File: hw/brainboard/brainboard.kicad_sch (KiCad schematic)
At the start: 0 parts

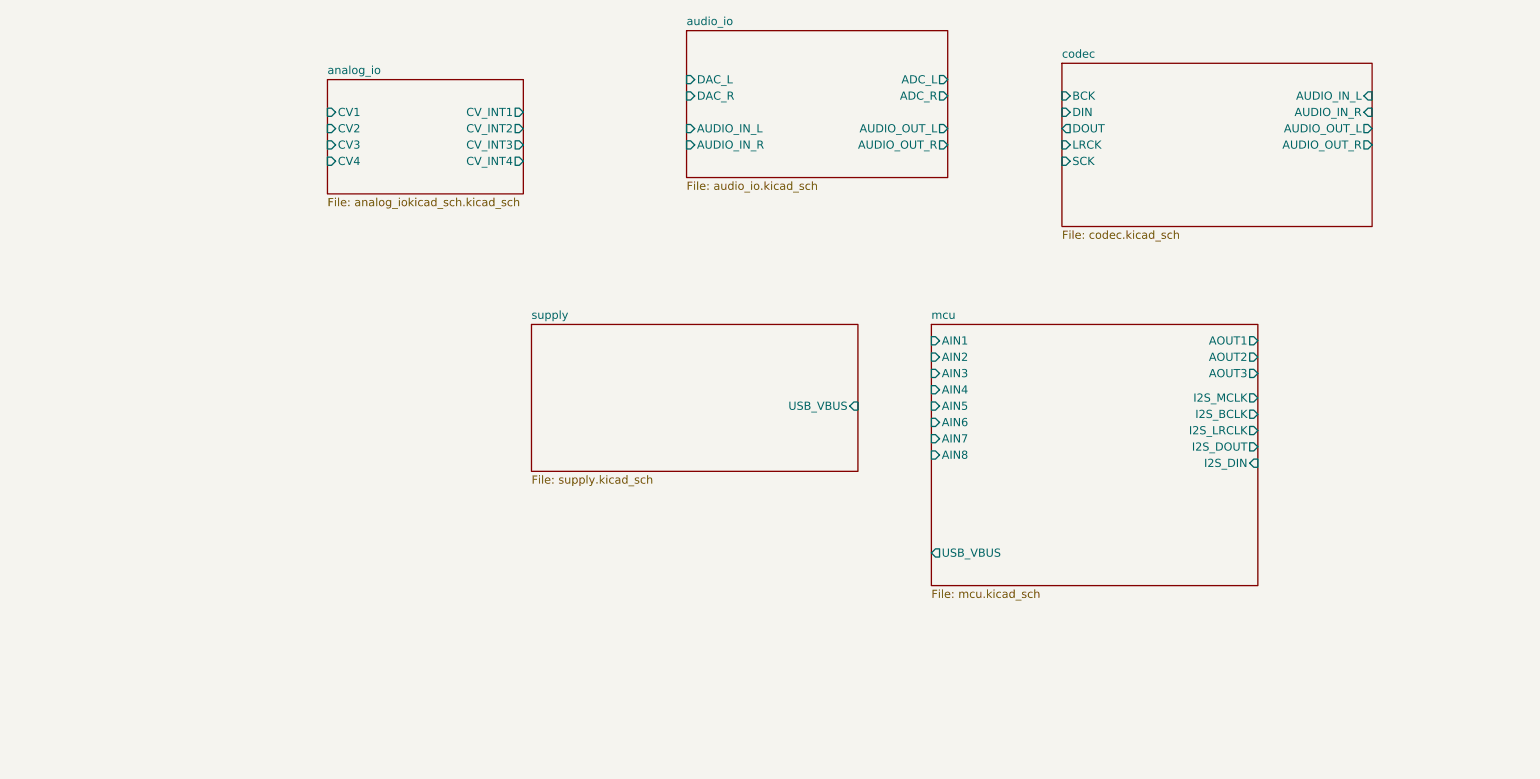
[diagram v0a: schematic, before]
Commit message: Laying out brains board
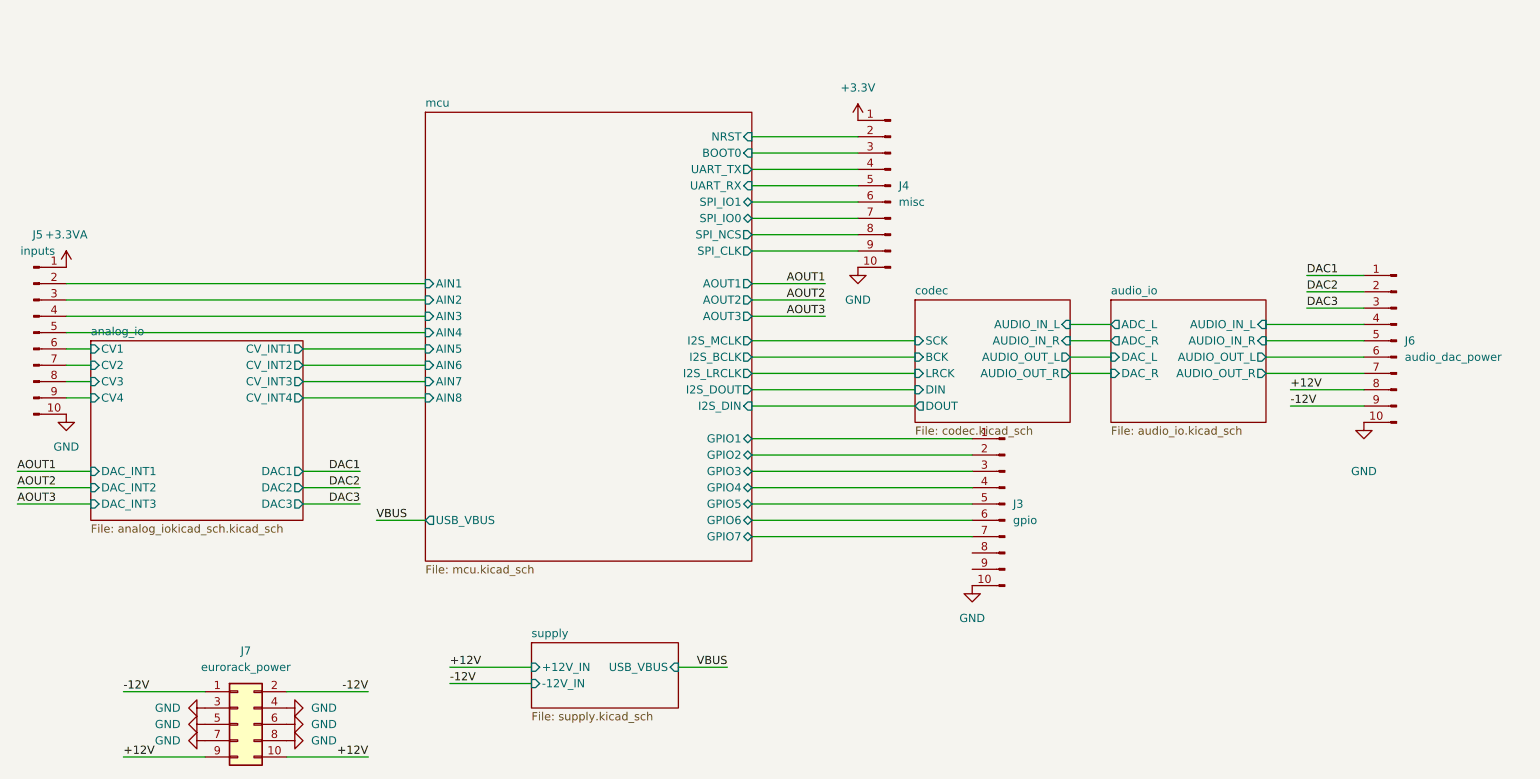
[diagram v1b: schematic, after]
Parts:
- added J3: gpio, Connector_PinHeader_2.54mm:PinHeader_1x10_P2.54mm_Vertical, symbol Connector:Conn_01x10_Pin
- added J4: misc, Connector_PinHeader_2.54mm:PinHeader_1x10_P2.54mm_Vertical, symbol Connector:Conn_01x10_Pin
- added J5: inputs, Connector_PinHeader_2.54mm:PinHeader_1x10_P2.54mm_Vertical, symbol Connector:Conn_01x10_Pin
- added J6: audio_dac_power, Connector_PinHeader_2.54mm:PinHeader_1x10_P2.54mm_Vertical, symbol Connector:Conn_01x10_Pin
- added J7: eurorack_power, Connector_IDC:IDC-Header_2x05_P2.54mm_Vertical, symbol Connector_Generic:Conn_02x05_Odd_Even
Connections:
- net analog_io/CV1: now also J5.6 (Pin_6)
- net analog_io/CV2: now also J5.7 (Pin_7)
- net analog_io/CV3: now also J5.8 (Pin_8)
- net analog_io/CV4: now also J5.9 (Pin_9)
- net audio_io/AUDIO_IN_L: now also J6.4 (Pin_4)
- net audio_io/AUDIO_IN_R: now also J6.5 (Pin_5)
- net audio_io/AUDIO_OUT_L: now also J6.6 (Pin_6)
- net audio_io/AUDIO_OUT_R: now also J6.7 (Pin_7)
- net mcu/AIN1: now also J5.2 (Pin_2)
- net mcu/AIN2: now also J5.3 (Pin_3)
- net mcu/AIN3: now also J5.4 (Pin_4)
- net mcu/AIN4: now also J5.5 (Pin_5)
- new net +12V: J6.8 (Pin_8), J7.10 (Pin_10), J7.9 (Pin_9)
- new net +3.3V: J4.1 (Pin_1)
- new net +3.3VA: J5.1 (Pin_1)
- new net -12V: J6.9 (Pin_9), J7.1 (Pin_1), J7.2 (Pin_2)
- new net DAC1: J6.1 (Pin_1)
- new net DAC2: J6.2 (Pin_2)
- new net DAC3: J6.3 (Pin_3)
- new net GND: J3.10 (Pin_10), J4.10 (Pin_10), J5.10 (Pin_10), J6.10 (Pin_10), J7.3 (Pin_3), J7.4 (Pin_4), J7.5 (Pin_5), J7.6 (Pin_6), J7.7 (Pin_7), J7.8 (Pin_8)
- new net mcu/BOOT0: J4.3 (Pin_3)
- new net mcu/GPIO1: J3.1 (Pin_1)
- new net mcu/GPIO2: J3.2 (Pin_2)
- new net mcu/GPIO3: J3.3 (Pin_3)
- new net mcu/GPIO4: J3.4 (Pin_4)
- new net mcu/GPIO5: J3.5 (Pin_5)
- new net mcu/GPIO6: J3.6 (Pin_6)
- new net mcu/GPIO7: J3.7 (Pin_7)
- new net mcu/NRST: J4.2 (Pin_2)
- new net mcu/SPI_CLK: J4.9 (Pin_9)
- new net mcu/SPI_IO0: J4.7 (Pin_7)
- new net mcu/SPI_IO1: J4.6 (Pin_6)
- new net mcu/SPI_NCS: J4.8 (Pin_8)
- new net mcu/UART_RX: J4.5 (Pin_5)
- new net mcu/UART_TX: J4.4 (Pin_4)
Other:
- sheet analog_io ports: added DAC1, DAC2, DAC3, DAC_INT1, DAC_INT2, DAC_INT3; removed none
- sheet mcu ports: added BOOT0, GPIO1, GPIO2, GPIO3, GPIO4, GPIO5, GPIO6, GPIO7, NRST, SPI_CLK, SPI_IO0, SPI_IO1, SPI_NCS, UART_RX, UART_TX; removed none
- sheet supply ports: added +12V_IN, -12V_IN; removed none
